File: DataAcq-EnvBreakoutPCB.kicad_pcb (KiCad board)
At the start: 4 copper layers, 21 parts, among them J1 ENV, U1 FS3000-1005, U2 MPL3115A2ST1, U3 SHT45

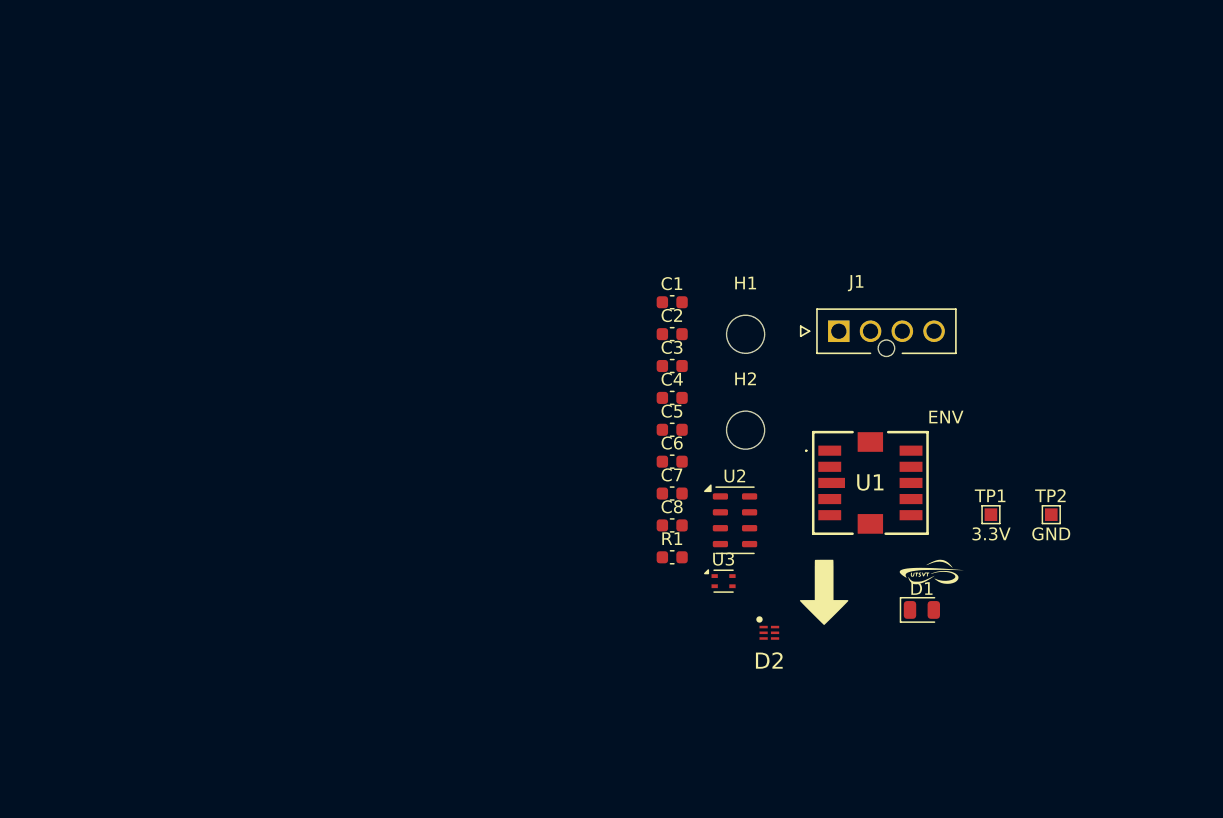
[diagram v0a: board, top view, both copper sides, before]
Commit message: layout kinda
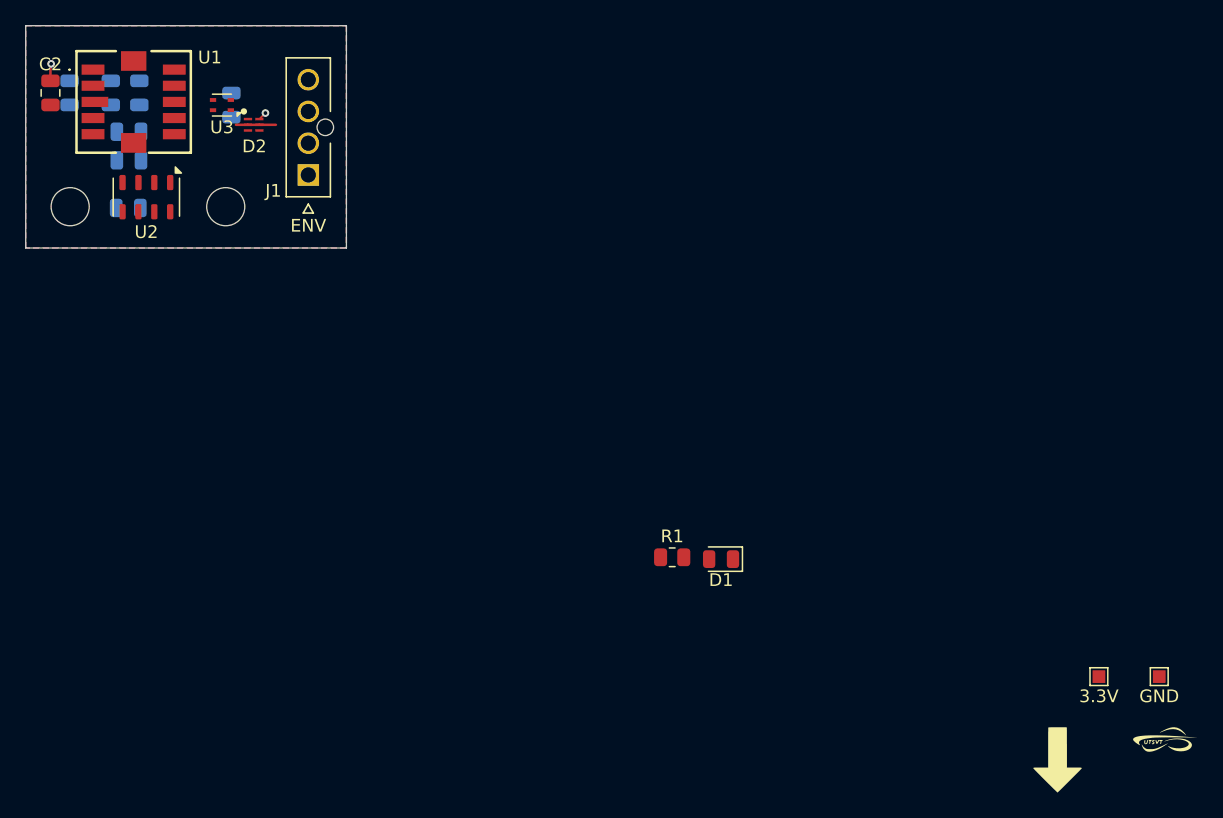
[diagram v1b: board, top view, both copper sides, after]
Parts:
- C1, C3, C4, C5, C6, C7, C8: footprint Capacitor_SMD:C_0603_1608Metric -> Capacitor_SMD:C_0805_2012Metric; moved to B.Cu
- C2: footprint Capacitor_SMD:C_0603_1608Metric -> Capacitor_SMD:C_0805_2012Metric
- R1: footprint Capacitor_SMD:C_0603_1608Metric -> Resistor_SMD:R_0805_2012Metric
- moved U1 65.3 mm to (105.0, 73.0)
- moved D2 57.0 mm to (114.5, 74.8)
- moved U3 54.5 mm to (112.0, 73.2), turned to 180 degrees
- moved H1 54.1 mm to (100.0, 81.2)
- moved U2 52.9 mm to (106.0, 80.5), turned to -90 degrees
- moved C8 52.8 mm to (104.6, 75.3)
- moved C2 52.5 mm to (98.5, 72.3), turned to -90 degrees
- moved C4 50.3 mm to (103.2, 72.3), turned to -90 degrees
- moved C1 50.2 mm to (100.0, 72.3), turned to -90 degrees
- moved C7 50.2 mm to (104.6, 77.6)
- moved C6 47.3 mm to (104.6, 81.3), turned to 180 degrees
- moved C3 47.1 mm to (105.5, 72.3), turned to 90 degrees
- moved H2 44.6 mm to (112.2, 81.2)
- moved J1 43.5 mm to (118.8, 78.8), turned to 90 degrees
- moved C5 43.1 mm to (112.7, 73.2), turned to -90 degrees
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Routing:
- net /I2C1_SCL: track 0.00 -> 4.10 mm, vias 0 -> 1
- net GND: track 0.00 -> 3.15 mm
- net +3.3V: track 0.00 -> 1.36 mm, vias 0 -> 1
- added copper zone on B.Cu, net +3.3V
- added copper zone on In1.Cu, net +3.3V
- added copper zone on F.Cu, net GND
- added copper zone on In2.Cu, net GND
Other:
- board outline added: 25.2 x 17.5 mm
- board text added: "STITCHING VIASSSSSS"
